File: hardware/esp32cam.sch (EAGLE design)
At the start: 32 parts, among them J1 MICRO_USB_B_HIROSE_ZX62-B-5PA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, J2 DM3AT-SF-PEJM5, SW1 TVAF06-A020B-R, X1 FA-238

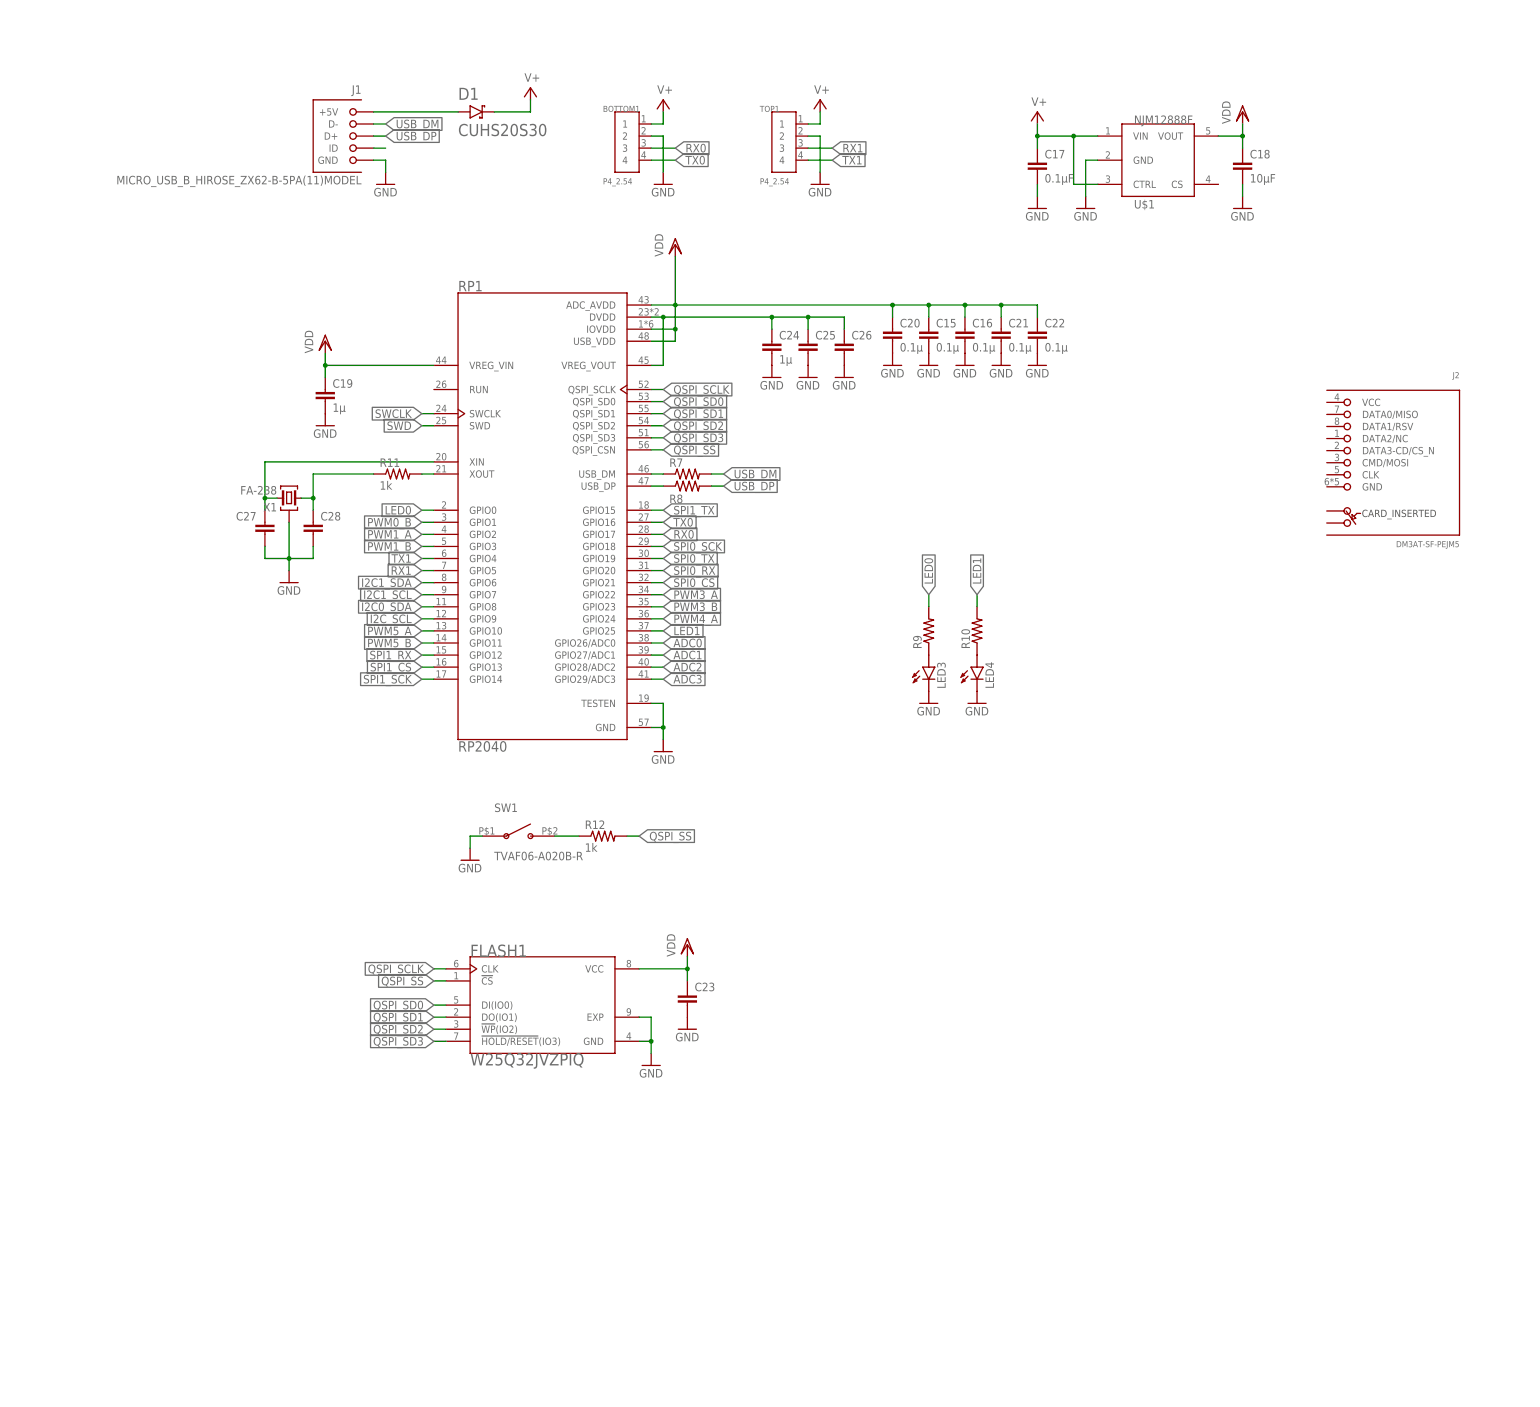
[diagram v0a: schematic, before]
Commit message: WIP
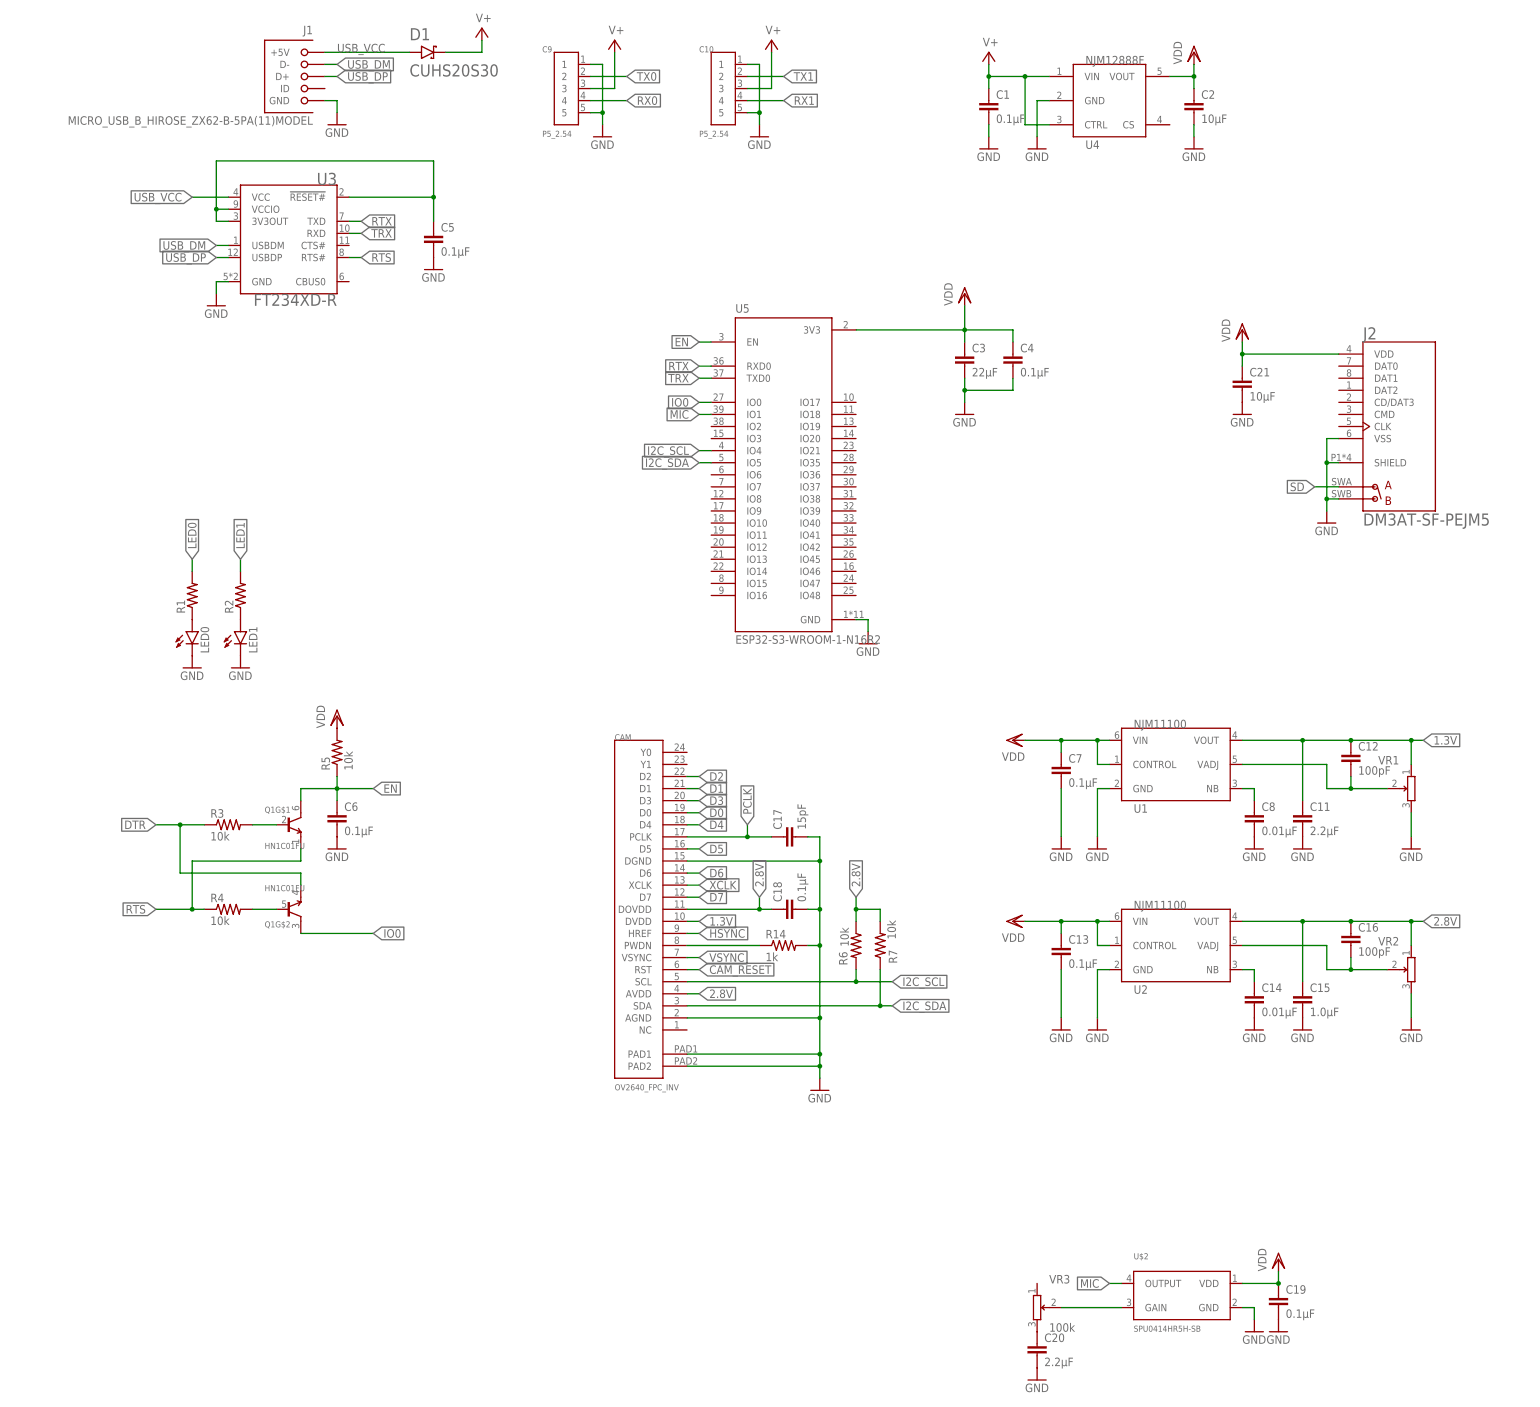
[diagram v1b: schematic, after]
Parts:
- removed BOTTOM1, TOP1: P4_2.54, pins:P4_2.54
- removed C22: 0.1µ, rcl:C-EUC0402
- removed C23, C25, C26, C27, C28: (no value), rcl:C-EUC0402
- removed C24: 1µ, rcl:C-EUC0402
- removed FLASH1: W25Q32JVZPIQ, W25Q32JVZPIQ:W25Q32JVZPIQ
- removed LED3, LED4: (no value), led:LEDCHIPLED_0603
- removed R10, R8, R9: (no value), rcl:R-US_R0402
- removed R11, R12: 1k, rcl:R-US_R0402
- removed RP1: RP2040, RP2040:RP2040
- removed SW1: TVAF06-A020B-R, switches:TVAF06-A020B-R
- removed U$1: NJM12888F, regulators:NJM12888F
- removed X1: FA-238, crystal':FA-238
- added C1, C13, C4, C5, C6, C7: 0.1µF, rcl:C-EUC0402
- added C10, C9: P5_2.54, pins:P5_2.54
- added C11: 2.2µF, rcl:C-EUC0402
- added C12: 100pF, rcl:C-EUC0402
- added C14, C8: 0.01µF, rcl:C-EUC0402
- added C2: 10µF, rcl:C-EUC0402
- added C3: 22µF, rcl:C-EUC0402
- added CAM: OV2640_FPC_INV, camera:OV2640_FPC_INV
- added LED0, LED1: (no value), led:LEDCHIPLED_0603
- added Q1: HN1C01FU, transistors:HN1C01FU
- added R1, R2: (no value), rcl:R-US_R0402
- added R14: 1k, rcl:R-US_R0402
- added R3, R4, R5, R6: 10k, rcl:R-US_R0402
- added U$2: SPU0414HR5H-SB, microphones:SPU0414HR5H-SB
- added U1, U2: NJM11100, regulators:NJM11100
- added U3: FT234XD-R, FT234XD-R:FT234XD-R
- added U4: NJM12888F, regulators:NJM12888F
- added U5: ESP32-S3-WROOM-1-N16R2, ESP32-S3-WROOM-1-N16R2:ESP32-S3-WROOM-1-N16R2
- added VR1, VR2: (no value), potentiometers:PVZ3A
- added VR3: 100k, potentiometers:PVZ3A
- C15: value 0.1µ -> 1.0µF
- C16: value 0.1µ -> 100pF
- C17: value 0.1µF -> 15pF
- C18: value 10µF -> 0.1µF
- C19: value 1µ -> 0.1µF
- C20: value 0.1µ -> 2.2µF
- C21: value 0.1µ -> 10µF
- J2: device connector:DM3AT-SF-PEJM5 -> dm3at-sf-pejm5:DM3AT-SF-PEJM5
- R7: value (none) -> 10k
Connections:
- removed net 1V2: C24.1, C25.1, C26.1, RP1.DVDD, RP1.VREG_VOUT
- removed net ADC0: RP1.GPIO26/ADC0
- removed net ADC1: RP1.GPIO27/ADC1
- removed net ADC2: RP1.GPIO28/ADC2
- removed net ADC3: RP1.GPIO29/ADC3
- removed net I2C0_SDA: RP1.GPIO8
- removed net I2C1_SCL: RP1.GPIO7
- removed net I2C1_SDA: RP1.GPIO6
- removed net N$12: R12.1, SW1.B
- removed net PWM0_B: RP1.GPIO1
- removed net PWM1_A: RP1.GPIO2
- removed net PWM1_B: RP1.GPIO3
- removed net PWM3_A: RP1.GPIO22
- removed net PWM3_B: RP1.GPIO23
- removed net PWM4_A: RP1.GPIO24
- removed net PWM5_A: RP1.GPIO10
- removed net PWM5_B: RP1.GPIO11
- removed net QSPI_SCLK: FLASH1.CLK, RP1.QSPI_SCLK
- removed net QSPI_SD0: FLASH1.DI(IO0), RP1.QSPI_SD0
- removed net QSPI_SD1: FLASH1.DO(IO1), RP1.QSPI_SD1
- removed net QSPI_SD2: FLASH1.!WP!(IO2), RP1.QSPI_SD2
- removed net QSPI_SD3: FLASH1.!HOLD/RESET!(IO3), RP1.QSPI_SD3
- removed net QSPI_SS: FLASH1.!CS, R12.2, RP1.QSPI_CSN
- removed net SPI0_CS: RP1.GPIO21
- removed net SPI0_RX: RP1.GPIO20
- removed net SPI0_SCK: RP1.GPIO18
- removed net SPI0_TX: RP1.GPIO19
- removed net SPI1_CS: RP1.GPIO13
- removed net SPI1_RX: RP1.GPIO12
- removed net SPI1_SCK: RP1.GPIO14
- removed net SPI1_TX: RP1.GPIO15
- removed net SWCLK: RP1.SWCLK
- removed net SWD: RP1.SWD
- removed net USB_DM_1: R7.1, RP1.USB_DM
- removed net USB_DP_1: R8.1, RP1.USB_DP
- removed net XIN1: C27.1, RP1.XIN, X1.2
- removed net XOUT1: R11.2, RP1.XOUT
- new net 1.3V: C11.1, C12.1, CAM.DVDD, U1.VOUT, VR1.1
- new net 2.8V: C15.1, C16.1, C18.1, CAM.AVDD, CAM.DOVDD, R6.1, R7.2, U2.VOUT, VR2.1
- new net CAM_RESET: CAM.RST
- new net D0: CAM.D0
- new net D1: CAM.D1
- new net D2: CAM.D2
- new net D3: CAM.D3
- new net D4: CAM.D4
- new net D5: CAM.D5
- new net D6: CAM.D6
- new net D7: CAM.D7
- new net DTR: Q1G$2.E, R3.1
- new net EN: C6.1, Q1G$1.C, R5.1, U5.EN
- new net HSYNC: CAM.HREF
- new net I2C_SDA: CAM.SDA, R7.1, U5.IO5
- new net IO0: Q1G$2.C, U5.IO0
- new net MIC: U$2.OUTPUT, U5.IO1
- new net N$1: C8.1, U1.NB
- new net N$13: U$2.GAIN, VR3.2
- new net N$14: C20.1, VR3.3
- new net N$2: C12.2, U1.VADJ, VR1.2
- new net N$3: C14.1, U2.NB
- new net N$4: C16.2, U2.VADJ, VR2.2
- new net N$7: LED0.A, R1.1
- new net PCLK: C17.1, CAM.PCLK
- new net RTS: Q1G$1.E, R4.1, U3.RTS#
- new net RTX: U3.TXD, U5.RXD0
- new net SD: J2.A
- new net TRX: U3.RXD, U5.TXD0
- new net USB_VCC: D1.A, J1.+5V, U3.VCC
- new net VSYNC: CAM.VSYNC
- new net XCLK: CAM.XCLK
- net GND: now also C1.2, C10.1, C10.5, C11.2, C13.2, C14.2, C2.2, C3.2, C4.2, C5.2, C6.2, C7.2, C8.2, C9.1, C9.5, CAM.AGND, CAM.DGND, CAM.PAD1, CAM.PAD2, J2.B, J2.SHIELD, J2.VSS, LED0.C, LED1.C, R14.2, U$2.GND, U1.GND, U2.GND, U3.GND, U4.GND, U5.GND, VR1.3, VR2.3; no longer BOTTOM1.2, C16.2, C22.2, C23.2, C24.2, C25.2, C26.2, C27.2, C28.2, FLASH1.EXP, FLASH1.GND, LED3.C, LED4.C, RP1.GND, RP1.TESTEN, SW1.A, TOP1.2, U$1.GND, X1.G
- net I2C_SCL: now also CAM.SCL, R6.2, U5.IO4; no longer RP1.GPIO9
- net LED0: now also R1.2; no longer R9.2, RP1.GPIO0
- net LED1: now also R2.2; no longer R10.2, RP1.GPIO25
- net N$10: now also CAM.PWDN, R14.1; no longer LED4.A, R10.1
- net N$11: now also Q1G$2.B, R4.2; no longer C28.1, R11.1, X1.1
- net N$6: now also C5.1, U3.!RESET#, U3.3V3OUT, U3.VCCIO; no longer J1.ID
- net N$8: now also LED1.A, R2.1; no longer D1.A, J1.+5V
- net N$9: now also Q1G$1.B, R3.2; no longer LED3.A, R9.1
- net RX0: now also C9.4; no longer BOTTOM1.3, RP1.GPIO17
- net RX1: now also C10.4; no longer RP1.GPIO5, TOP1.3
- net TX0: now also C9.2; no longer BOTTOM1.4, RP1.GPIO16
- net TX1: now also C10.2; no longer RP1.GPIO4, TOP1.4
- net USB_DM: now also U3.USBDM; no longer R7.2
- net USB_DP: now also U3.USBDP; no longer R8.2
- net V+: now also C1.1, C10.3, C9.3, U4.CTRL, U4.VIN; no longer BOTTOM1.1, C17.1, TOP1.1, U$1.CTRL, U$1.VIN
- net VDD: now also C13.1, C2.1, C3.1, C4.1, C7.1, J2.VDD, R5.2, U$2.VDD, U1.CONTROL, U1.VIN, U2.CONTROL, U2.VIN, U4.VOUT, U5.3V3; no longer C15.1, C16.1, C18.1, C20.1, C22.1, C23.1, FLASH1.VCC, RP1.ADC_AVDD, RP1.IOVDD, RP1.USB_VDD, RP1.VREG_VIN, U$1.VOUT
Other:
- moved on the sheet: C15, C16, C17, C18, C19, C20, C21, D1, J1, R7
